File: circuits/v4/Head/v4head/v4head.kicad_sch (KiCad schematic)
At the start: 13 parts, among them J1 Raspberry_Pi_2_3

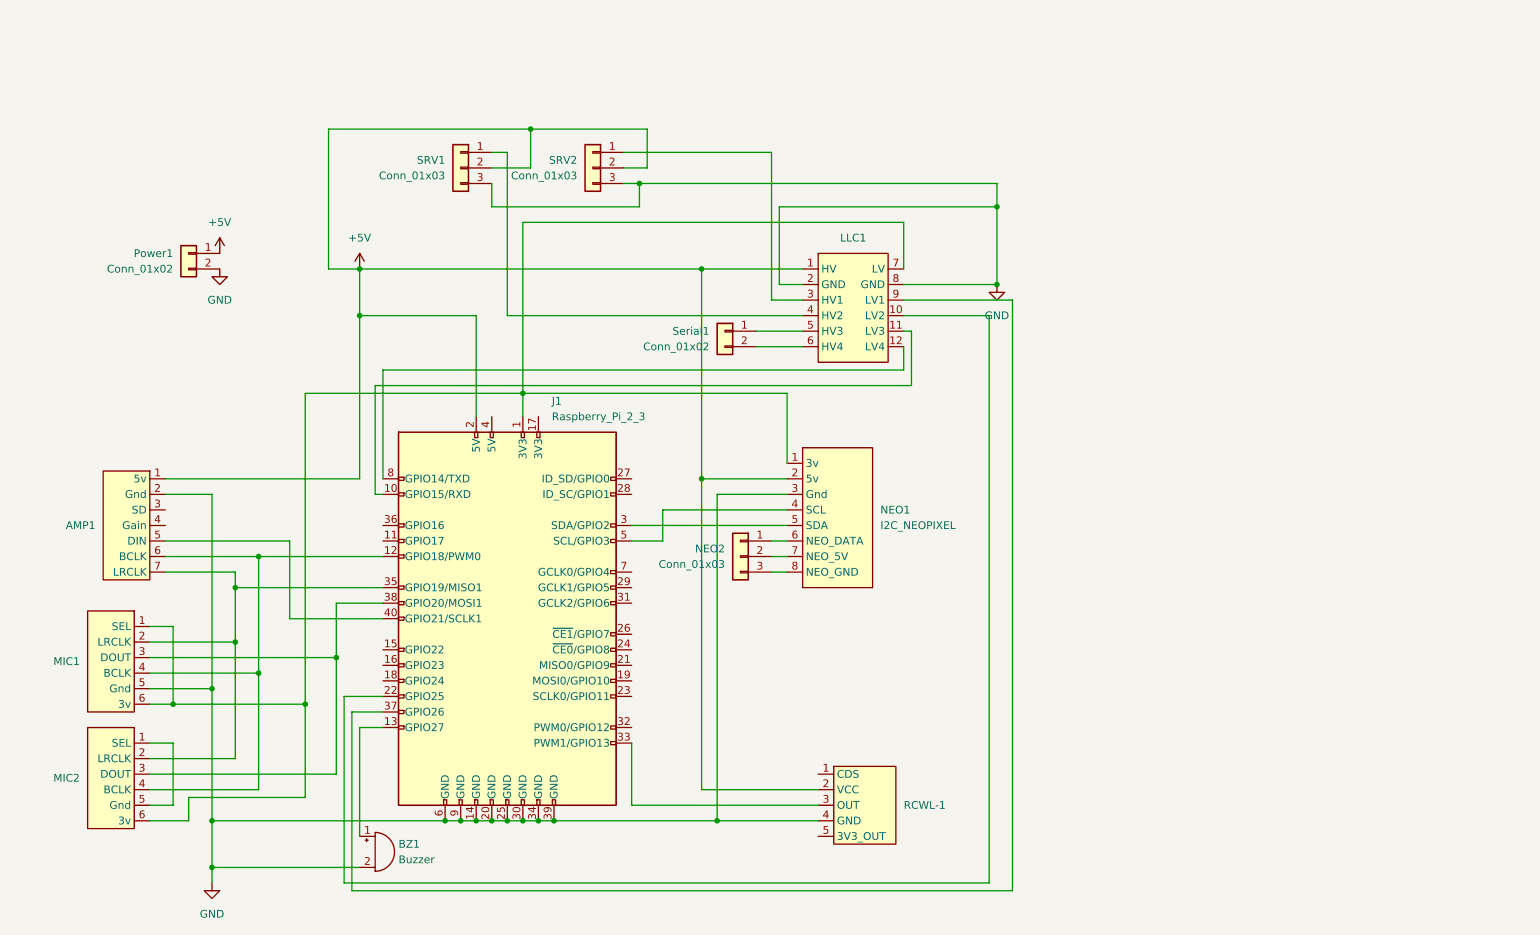
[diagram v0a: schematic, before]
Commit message: Updates
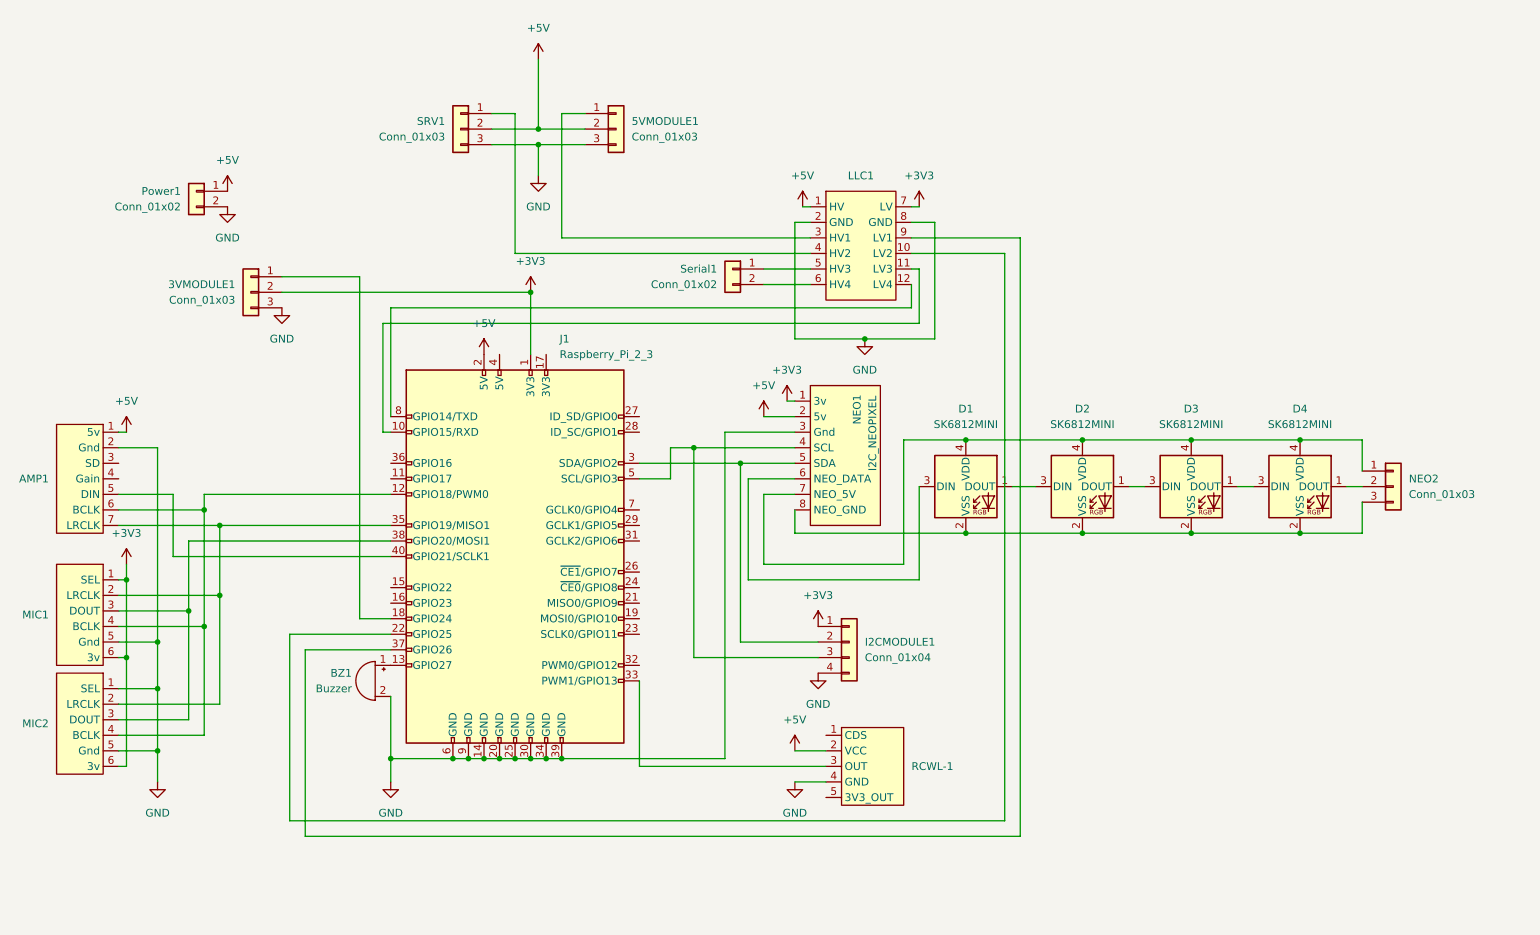
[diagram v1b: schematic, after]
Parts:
- added 3VMODULE1: Conn_01x03, Connector_JST:JST_EH_B3B-EH-A_1x03_P2.50mm_Vertical, symbol Connector_Generic:Conn_01x03
- added D1, D2, D3, D4: SK6812MINI, LED_SMD:LED_SK6812MINI_PLCC4_3.5x3.5mm_P1.75mm, symbol LED:SK6812MINI
- added I2CMODULE1: Conn_01x04, Connector_JST:JST_EH_B4B-EH-A_1x04_P2.50mm_Vertical, symbol Connector_Generic:Conn_01x04
- 5VMODULE1: renamed from SRV2; footprint Connector_Wire:SolderWire-0.1sqmm_1x03_P3.6mm_D0.4mm_OD1mm -> Connector_JST:JST_EH_B3B-EH-A_1x03_P2.50mm_Vertical
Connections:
- net GND: now also MIC2.1 (SEL), MIC2.5 (Gnd), 3VMODULE1.3 (Pin_3), I2CMODULE1.4 (Pin_4)
- net +3V3: now reaches J1.1 (3V3), LLC1.7 (LV), MIC1.1 (SEL), MIC1.6 (3v), MIC2.6 (3v), NEO1.1 (3v)
- net +3V3: now also 3VMODULE1.2 (Pin_2), I2CMODULE1.1 (Pin_1)
- net at NEO2.1 (Pin_1): now also NEO1.7 (NEO_5V), D1.4 (VDD), D2.4 (VDD), D3.4 (VDD), D4.4 (VDD); no longer NEO1.6 (NEO_DATA)
- net at NEO2.2 (Pin_2): now also D4.1 (DOUT); no longer NEO1.7 (NEO_5V)
- net at NEO1.8 (NEO_GND), NEO2.3 (Pin_3): now also D1.2 (VSS), D2.2 (VSS), D3.2 (VSS), D4.2 (VSS)
- net at J1.18 (GPIO24): now also 3VMODULE1.1 (Pin_1)
- net at J1.3 (SDA/GPIO2), NEO1.5 (SDA): now also I2CMODULE1.2 (Pin_2)
- net at J1.5 (SCL/GPIO3), NEO1.4 (SCL): now also I2CMODULE1.3 (Pin_3)
- new net: D3.1 (DOUT), D4.3 (DIN)
- new net: D1.1 (DOUT), D2.3 (DIN)
- new net: D1.3 (DIN), NEO1.6 (NEO_DATA)
- new net: D2.1 (DOUT), D3.3 (DIN)
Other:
- title: (none) -> Modular Biped Head Pi Connector
- moved on the sheet: 5VMODULE1, AMP1, BZ1, J1, LLC1, MIC1, MIC2, NEO1, NEO2, Power1, RCWL-1, SRV1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

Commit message: Updates
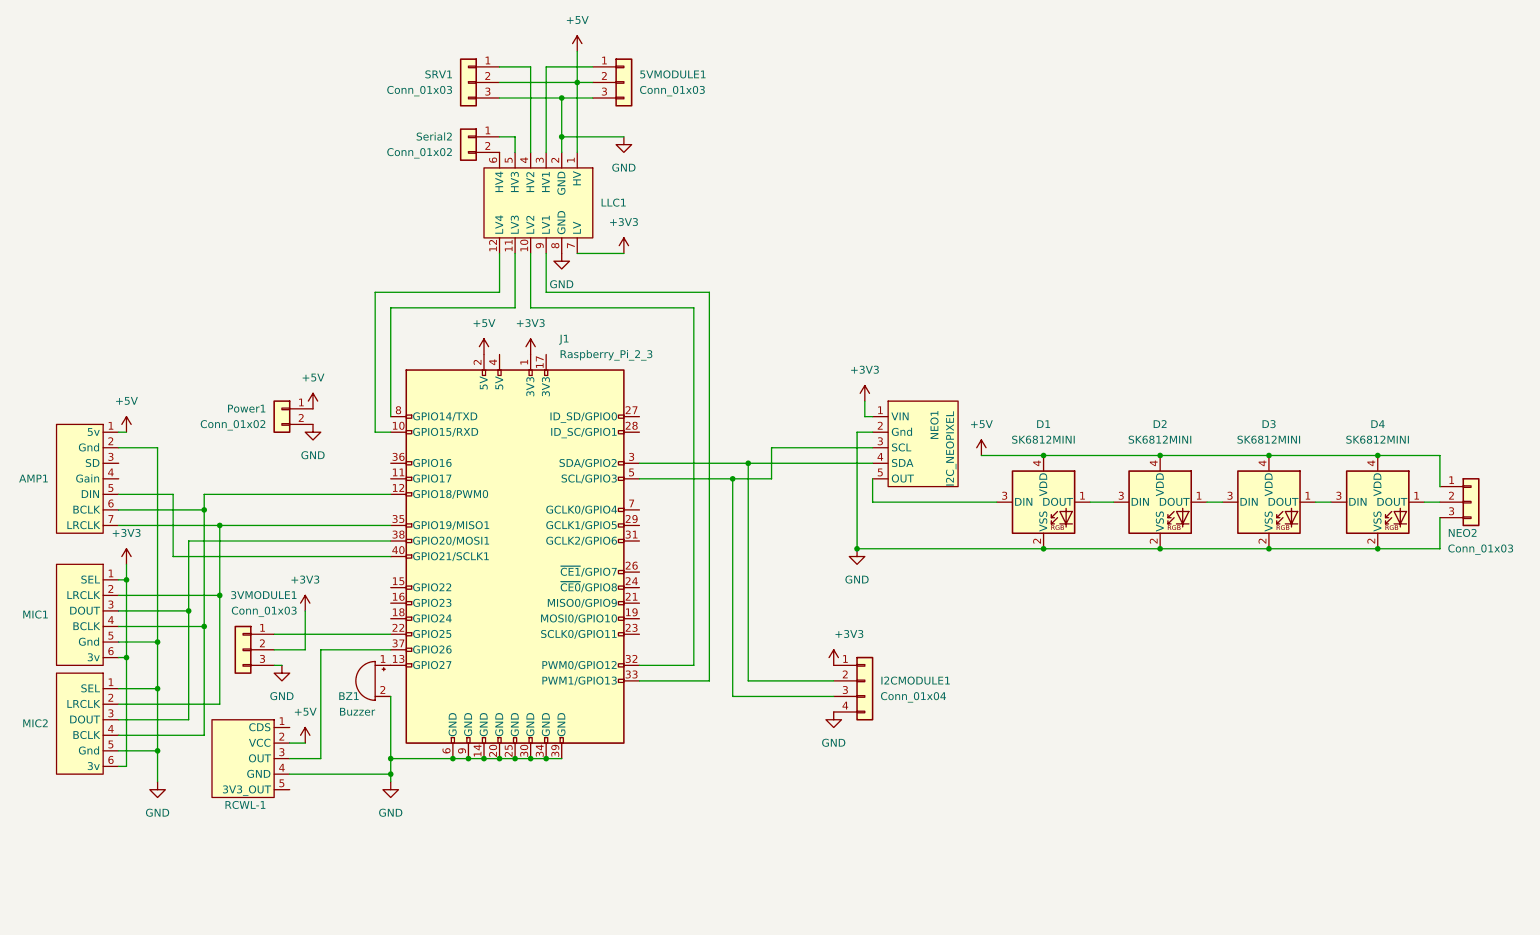
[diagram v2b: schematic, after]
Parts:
- removed Serial1: Conn_01x02, Connector_JST:JST_EH_B2B-EH-A_1x02_P2.50mm_Vertical, symbol Connector_Generic:Conn_01x02
- added Serial2: Conn_01x02, Connector_JST:JST_XH_B2B-XH-A_1x02_P2.50mm_Vertical, symbol Connector_Generic:Conn_01x02
- 3VMODULE1, 5VMODULE1, NEO2: footprint Connector_JST:JST_EH_B3B-EH-A_1x03_P2.50mm_Vertical -> Connector_JST:JST_XH_B3B-XH-A_1x03_P2.50mm_Vertical
- I2CMODULE1: footprint Connector_JST:JST_EH_B4B-EH-A_1x04_P2.50mm_Vertical -> Connector_JST:JST_XH_B4B-XH-A_1x04_P2.50mm_Vertical
- J1: footprint Connector_JST:JST_PUD_S40B-PUDSS-1_2x20_P2.00mm_Horizontal -> Connector_PinHeader_2.54mm:PinHeader_2x20_P2.54mm_Vertical
- Power1: footprint Connector_JST:JST_EH_B2B-EH-A_1x02_P2.50mm_Vertical -> Connector_JST:JST_XH_B2B-XH-A_1x02_P2.50mm_Vertical
- SRV1: footprint Connector_Wire:SolderWire-0.1sqmm_1x03_P3.6mm_D0.4mm_OD1mm -> Connector_PinHeader_2.54mm:PinHeader_1x03_P2.54mm_Vertical
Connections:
- net +5V: now also D1.4 (VDD), D2.4 (VDD), D3.4 (VDD), D4.4 (VDD), NEO2.1 (Pin_1); no longer NEO1.2 (5v)
- net GND: now also D1.2 (VSS), D2.2 (VSS), D3.2 (VSS), D4.2 (VSS), NEO1.2 (Gnd), NEO2.3 (Pin_3); no longer NEO1.3 (Gnd)
- net at RCWL-1.3 (OUT): now also J1.37 (GPIO26); no longer J1.33 (PWM1/GPIO13)
- net at D1.3 (DIN): now also NEO1.5 (OUT); no longer NEO1.6 (NEO_DATA)
- net at 3VMODULE1.1 (Pin_1): now also J1.22 (GPIO25); no longer J1.18 (GPIO24)
- net at J1.10 (GPIO15/RXD): now also LLC1.12 (LV4); no longer LLC1.11 (LV3)
- net at LLC1.10 (LV2): now also J1.32 (PWM0/GPIO12); no longer J1.22 (GPIO25)
- net at I2CMODULE1.2 (Pin_2), J1.3 (SDA/GPIO2): now also NEO1.4 (SDA); no longer NEO1.5 (SDA)
- net at LLC1.9 (LV1): now also J1.33 (PWM1/GPIO13); no longer J1.37 (GPIO26)
- net at I2CMODULE1.3 (Pin_3), J1.5 (SCL/GPIO3): now also NEO1.3 (SCL); no longer NEO1.4 (SCL)
- net at J1.8 (GPIO14/TXD): now also LLC1.11 (LV3); no longer LLC1.12 (LV4)
- net at LLC1.5 (HV3): now also Serial2.1 (Pin_1)
- net at LLC1.6 (HV4): now also Serial2.2 (Pin_2)
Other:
- moved on the sheet: 3VMODULE1, 5VMODULE1, D1, D2, D3, D4, I2CMODULE1, LLC1, NEO2, Power1, RCWL-1, SRV1
